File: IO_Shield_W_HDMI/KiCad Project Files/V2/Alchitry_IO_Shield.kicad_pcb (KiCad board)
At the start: 4 copper layers, 65 x 45 mm, 76 parts, among them Q1 FDN340P, Q2 FDN340P, Q3 FDN340P, Q4 FDN340P, SW1 SW_DIP_x08, SW2 SW_DIP_x08, U1 Alchitry_Single

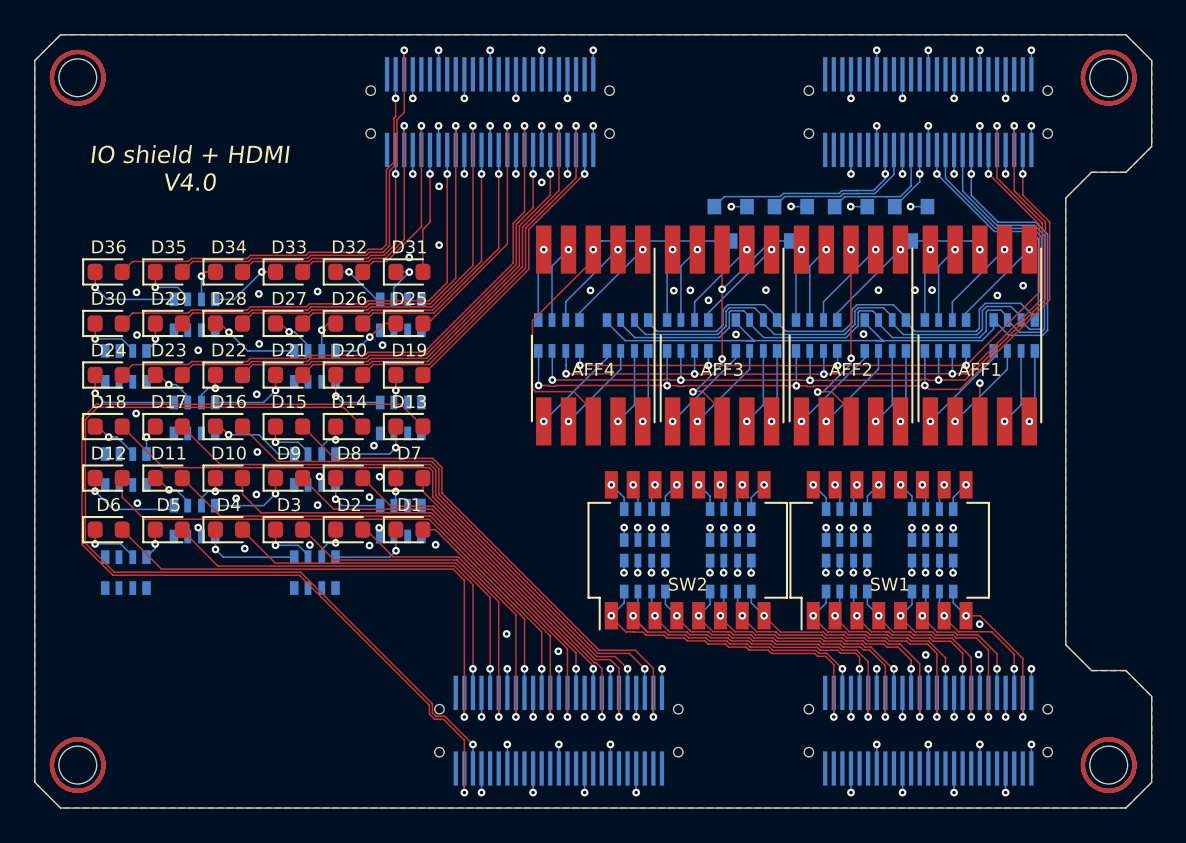
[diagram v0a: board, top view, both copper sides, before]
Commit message: layout again
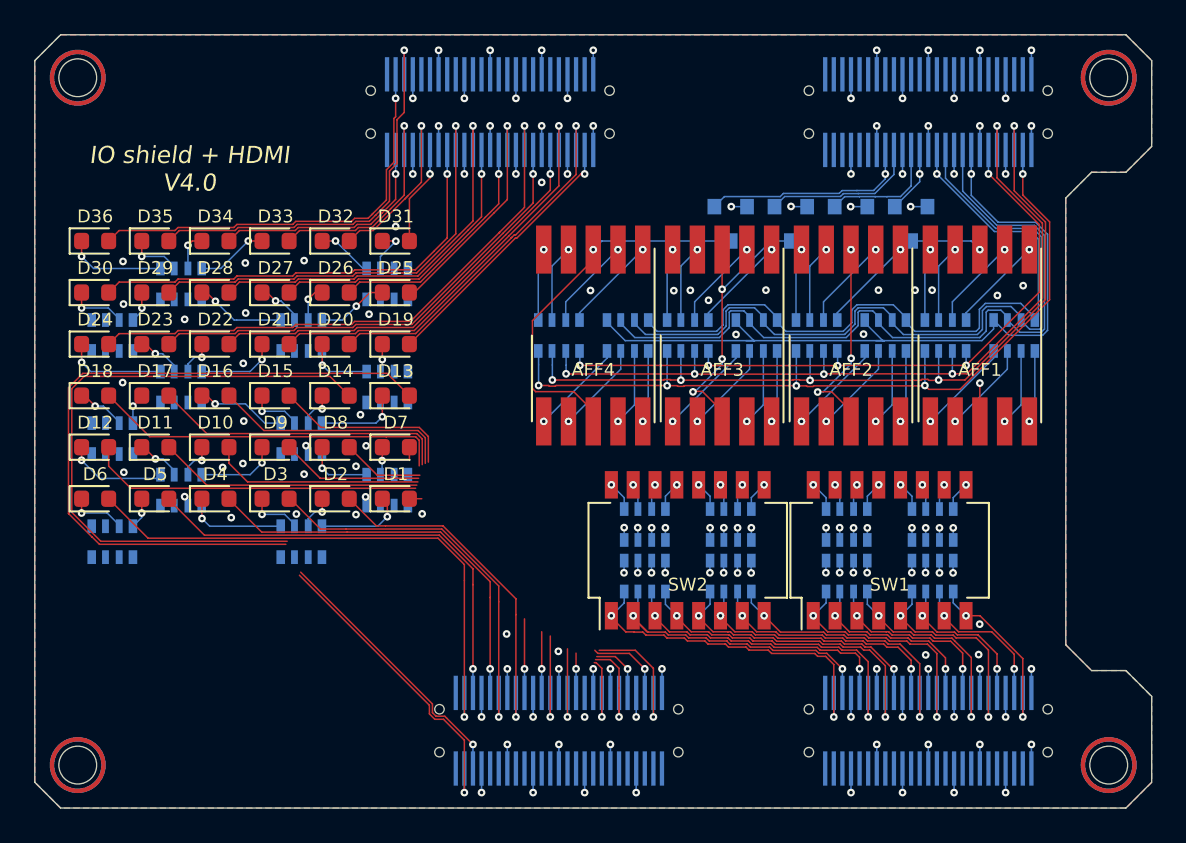
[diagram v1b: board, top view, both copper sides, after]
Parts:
- moved D20 1.96 mm to (29.5, 30.0)
- moved D21 1.96 mm to (26.0, 30.0)
- moved D22 1.96 mm to (22.5, 30.0)
- moved D23 1.96 mm to (19.0, 30.0)
- moved D24 1.96 mm to (15.5, 30.0)
- moved D26 1.96 mm to (29.5, 27.0)
- moved D27 1.96 mm to (26.0, 27.0)
- moved D28 1.96 mm to (22.5, 27.0)
- moved D29 1.96 mm to (19.0, 27.0)
- moved D30 1.96 mm to (15.5, 27.0)
- moved D32 1.96 mm to (29.5, 24.0)
- moved D33 1.96 mm to (26.0, 24.0)
- moved D34 1.96 mm to (22.5, 24.0)
- moved D35 1.96 mm to (19.0, 24.0)
- moved D36 1.96 mm to (15.5, 24.0)
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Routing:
- net /LED6: track 19.7 -> 5.62 mm
- net /LED17: track 39.9 -> 26.5 mm
- net /LED16: track 34.1 -> 20.8 mm
- net /LED7: track 19.5 -> 6.39 mm
- net /LED14: track 31.4 -> 18.4 mm
- net /LED15: track 31.6 -> 18.7 mm
- net /LED8: track 22.5 -> 10.6 mm
- net /LED9: track 29.0 -> 17.8 mm
- net /LED10: track 31.4 -> 21.5 mm
- net /LED11: track 32.4 -> 23.1 mm
- net /LED0: track 12.4 -> 5.07 mm
- net /LED1: track 18.2 -> 20.4 mm
- net /LED2: track 21.2 -> 23.3 mm
- net /LED3: track 21.6 -> 23.7 mm
- net /LED4: track 24.6 -> 26.6 mm
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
